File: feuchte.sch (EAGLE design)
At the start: 33 parts, among them CON1 CON_PCB_7.5MM_3-POLE, CON2 CON_PCB_7.5MM_3-POLE, IC1 IC_ATMEGA32U2-AU, IC2 ESD_USB_IP4234CZ6, IC3 IC_ULN2003AD, K1 RELAY_G5LA, K2 RELAY_G5LA, Q1 16MHz

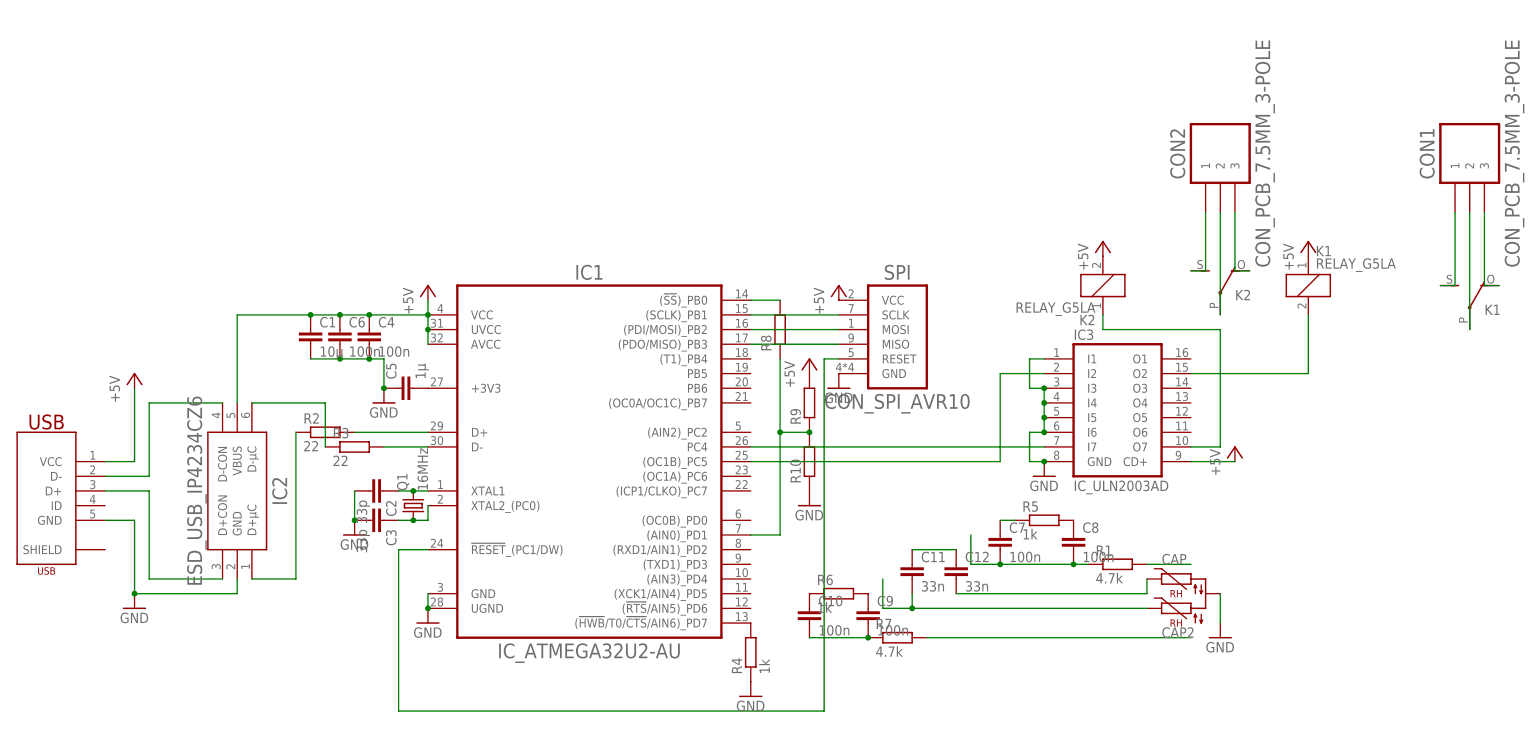
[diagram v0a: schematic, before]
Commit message: Layout geschätzt bei 80%
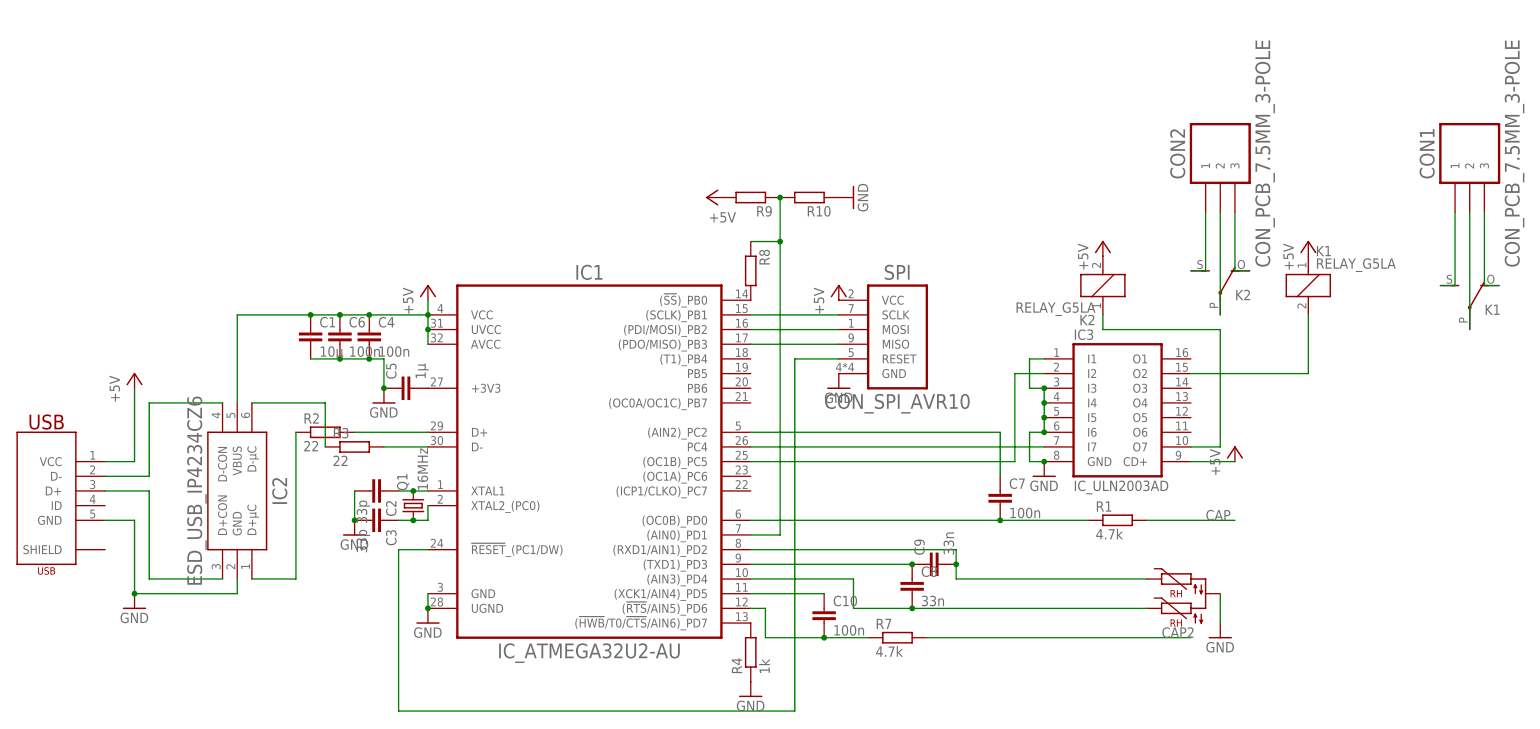
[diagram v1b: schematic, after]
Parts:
- removed C11, C12: 33n, Bauelemente:C
- removed R5, R6: 1k, Bauelemente:RSMD
- C8, C9: value 100n -> 33n
- R10, R9: device Bauelemente:RTHT -> Bauelemente:RTHT_7.5MM
- R8: device Bauelemente:RTHT -> Bauelemente:RTHT_10MM
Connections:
- removed net N$23: C12.2, U$2.3
- removed net N$26: C9.1, R6.2
- removed net N$28: C10.2, C9.2, R7.1
- new net N$22: C9.2, IC1.(RXD1/AIN1)_PD2, U$2.3
- net N$10: now also C10.1, IC1.(XCK1/AIN4)_PD5; no longer C8.1, R5.2
- net N$24: now also C8.1, C9.1, IC1.(TXD1)_PD3; no longer C11.1, C12.1
- net N$25: now also C8.2, IC1.(AIN3)_PD4; no longer C11.2
- net N$27: now also C10.2, IC1.(!RTS!/AIN5)_PD6, R7.1; no longer C10.1, R6.1
- net N$8: now also IC1.(AIN2)_PC2; no longer R5.1
- net N$9: now also IC1.(OC0B)_PD0; no longer C8.2
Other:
- moved on the sheet: C10, C7, C8, C9, R1, R10, R8, R9

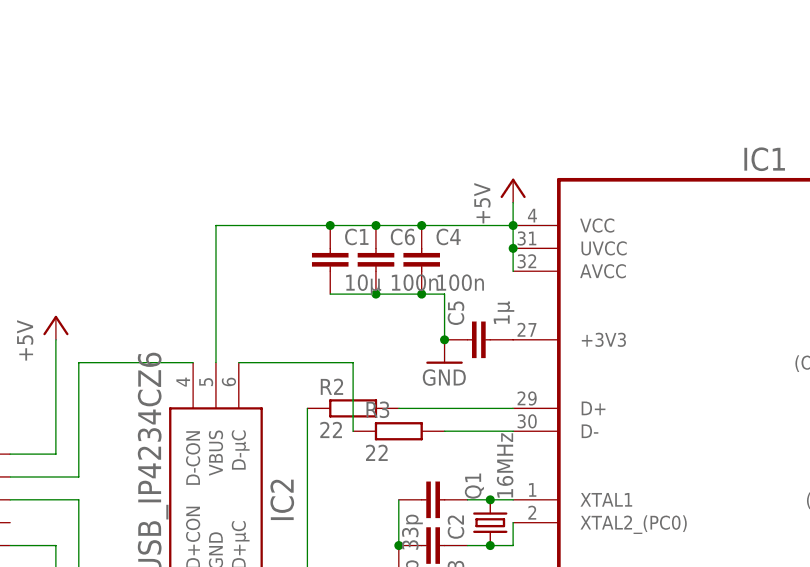
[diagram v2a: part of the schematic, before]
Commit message: Layout V1 fertig
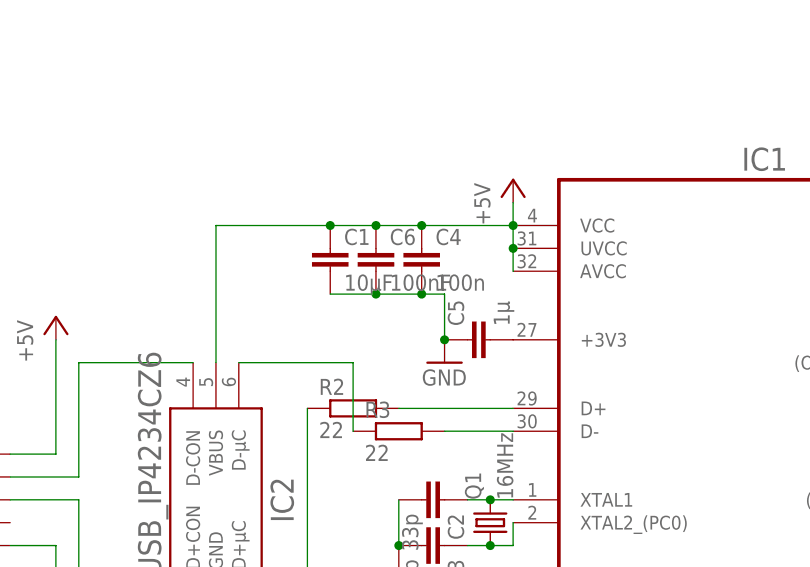
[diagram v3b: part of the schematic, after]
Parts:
- C1: value 10µ -> 10µF
- C6: value 100n -> 100nF
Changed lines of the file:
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@@
 <part name="IC3" library="Bauelemente" deviceset="IC_ULN2003A" device="D"/>
 <part name="R1" library="Bauelemente" deviceset="R" device="SMD" value="4.7k"/>
-<part name="C1" library="Bauelemente" deviceset="C" device="" value="10µ"/>
+<part name="C1" library="Bauelemente" deviceset="C" device="" value="10µF"/>
 <part name="C2" library="Bauelemente" deviceset="C" device="" value="33p"/>
 <part name="C3" library="Bauelemente" deviceset="C" device="" value="33p"/>
 <part name="C4" library="Bauelemente" deviceset="C" device="" value="100n"/>
 <part name="C5" library="Bauelemente" deviceset="C" device="" value="1µ"/>
-<part name="C6" library="Bauelemente" deviceset="C" device="" value="100n"/>
+<part name="C6" library="Bauelemente" deviceset="C" device="" value="100nF"/>
 <part name="R2" library="Bauelemente" deviceset="R" device="SMD" value="22"/>
 <part name="R3" library="Bauelemente" deviceset="R" device="SMD" value="22"/>
